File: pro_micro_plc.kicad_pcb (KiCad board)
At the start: 2 copper layers, 75 x 50 mm, 40 parts, among them J1 Conn_01x06_Pin, J2 Conn_01x02_Socket, J3 Conn_01x02_Socket, J4 Conn_01x02_Socket, J5 Conn_01x02_Pin, J6 Conn_01x04_Pin, J7 Conn_01x04_Pin, Q1 2N7002K, Q2 2N7002K, Q3 2N7002K, Q4 2N7002K, U1 Sparkfun_Pro_Micro, U2 PC817, U3 PC817, U4 PC817, U5 PC817, U6 MAX485E

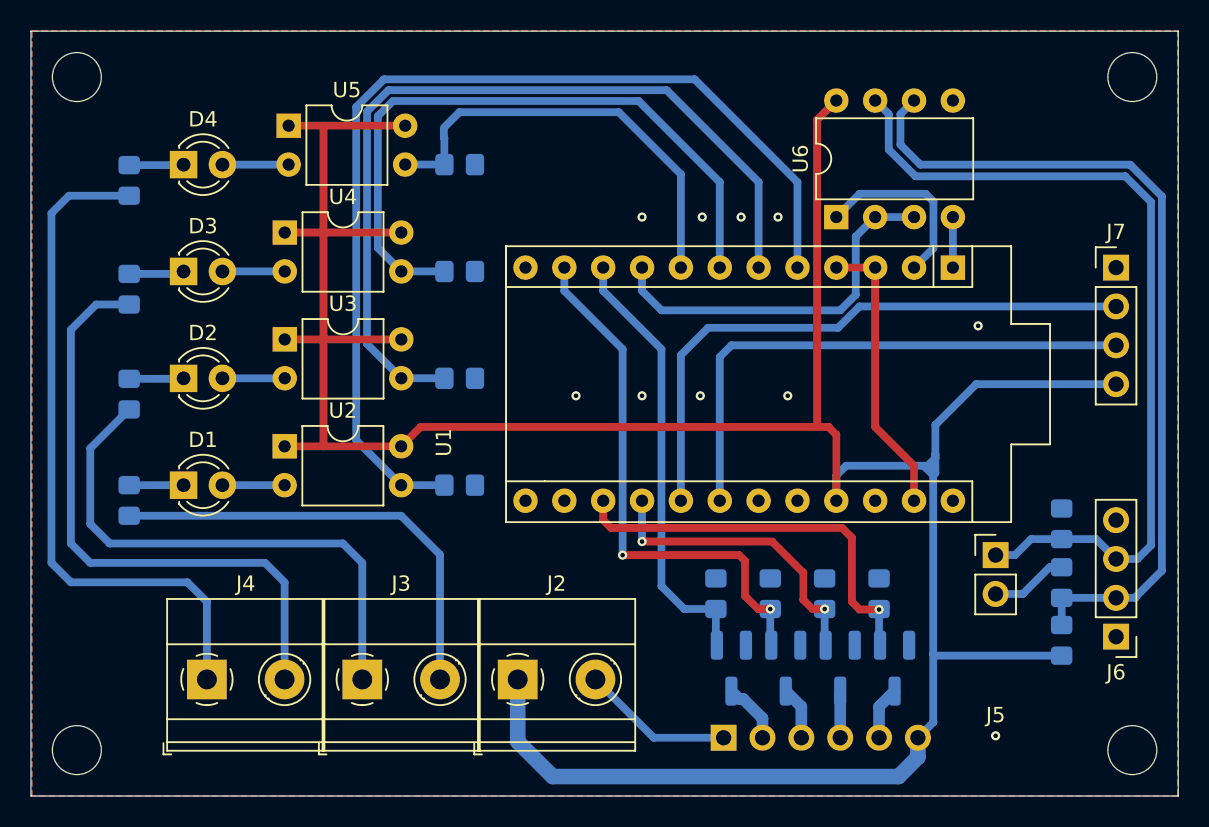
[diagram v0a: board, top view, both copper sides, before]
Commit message: smallest PCB
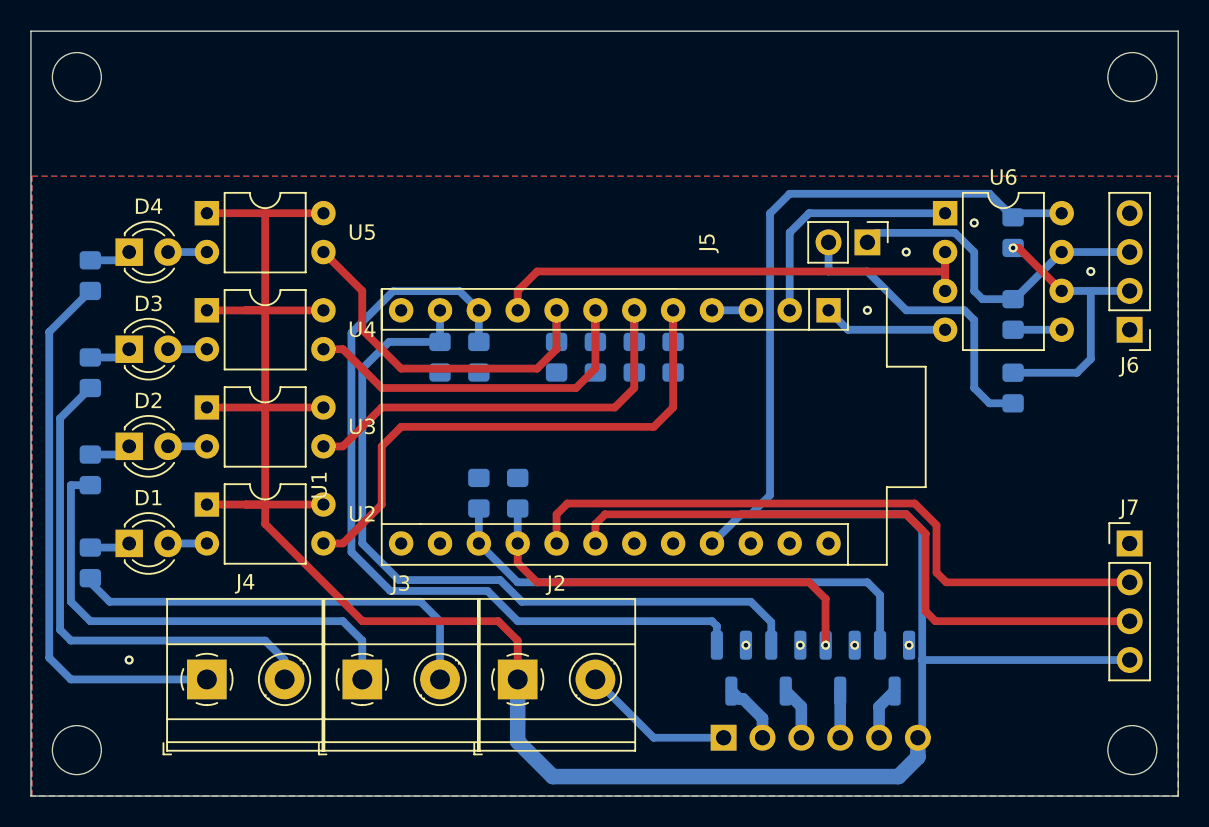
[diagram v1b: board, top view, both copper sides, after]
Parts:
- moved R1 27.0 mm to (71.6, 48.8)
- moved R15 26.8 mm to (106.6, 31.8), turned to 90 degrees
- moved R3 26.6 mm to (69.1, 39.9), turned to 90 degrees
- moved J5 22.1 mm to (97.0, 32.4), turned to -90 degrees
- moved R4 21.9 mm to (71.6, 39.9), turned to 90 degrees
- moved R2 21.1 mm to (74.2, 48.8)
- moved J6 20.1 mm to (114.2, 38.1)
- moved J7 18.1 mm to (114.2, 52.1)
- moved R5 16.3 mm to (84.3, 39.9), turned to -90 degrees
- moved R8 14.1 mm to (76.7, 39.9), turned to -90 degrees
- moved R14 14.0 mm to (106.6, 37.1), turned to 90 degrees
- moved R9 13.1 mm to (106.6, 41.9), turned to -90 degrees
- moved R6 11.5 mm to (81.8, 39.9), turned to -90 degrees
- moved R7 10.5 mm to (79.2, 39.9), turned to -90 degrees
- moved U1 8.59 mm to (66.5, 52.1)
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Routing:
- net /Bus+: track 55.3 -> 18.7 mm, vias 0 -> 1
- net /Bus-: track 56.1 -> 22.0 mm
- net /IX0.0: track 66.7 -> 37.2 mm
- net /IX0.1: track 55.4 -> 29.0 mm
- net /QX0.0: track 28.5 -> 53.5 mm
- net /IX0.2: track 44.2 -> 25.2 mm
- net Net-(J5-Pin_2): track 5.04 -> 20.1 mm
- net /QX0.1: track 35.0 -> 49.7 mm, vias 2 -> 0
- net GND: track 28.8 -> 15.7 mm, vias 10 -> 9
- net /DE: track 24.6 -> 34.8 mm
- net Net-(J4-Pin_1): track 44.8 -> 36.0 mm
- net /QX0.3: track 20.4 -> 27.7 mm, vias 2 -> 1
- net /IW0.1: track 35.6 -> 42.3 mm
- net /QX0.2: track 26.6 -> 33.2 mm, vias 1 -> 0
- net Net-(J4-Pin_2): track 40.0 -> 33.4 mm
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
